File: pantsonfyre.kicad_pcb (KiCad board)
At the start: 2 copper layers, 27 parts, among them J1 3.5mm TRRS, J2 USB_C_Receptacle, SW1 SW_Push, SW2 SW_Push, SW3 SW_Push, U1 CAP1206-x-SL, U2 STM32C011J4Mx, U3 MCP4725xxx-xCH, U4 CAP1206-x-SL, U5 CAP1206-x-SL, U7 AMS1117-3.3, U8 PAM8302AAD

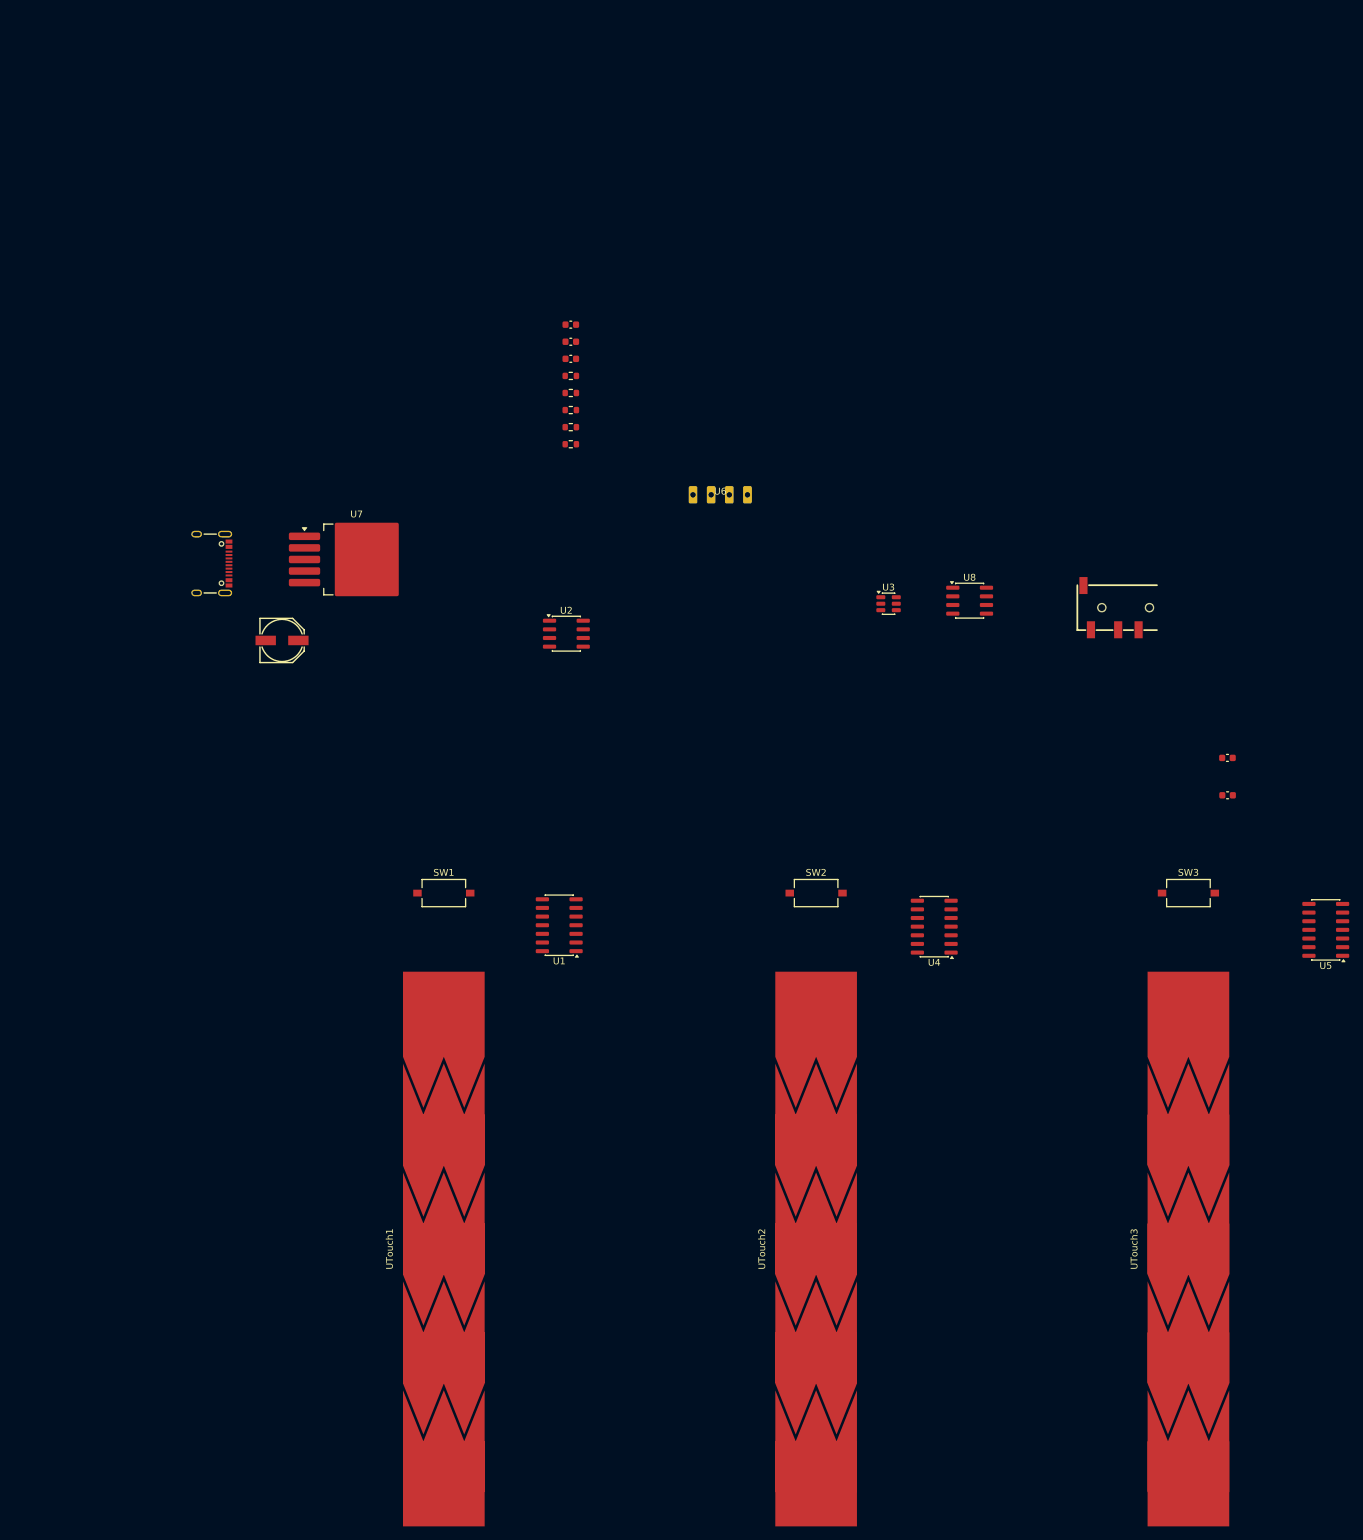
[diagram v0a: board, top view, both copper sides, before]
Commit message: Did lots of stuff + removed the custom footprint for header
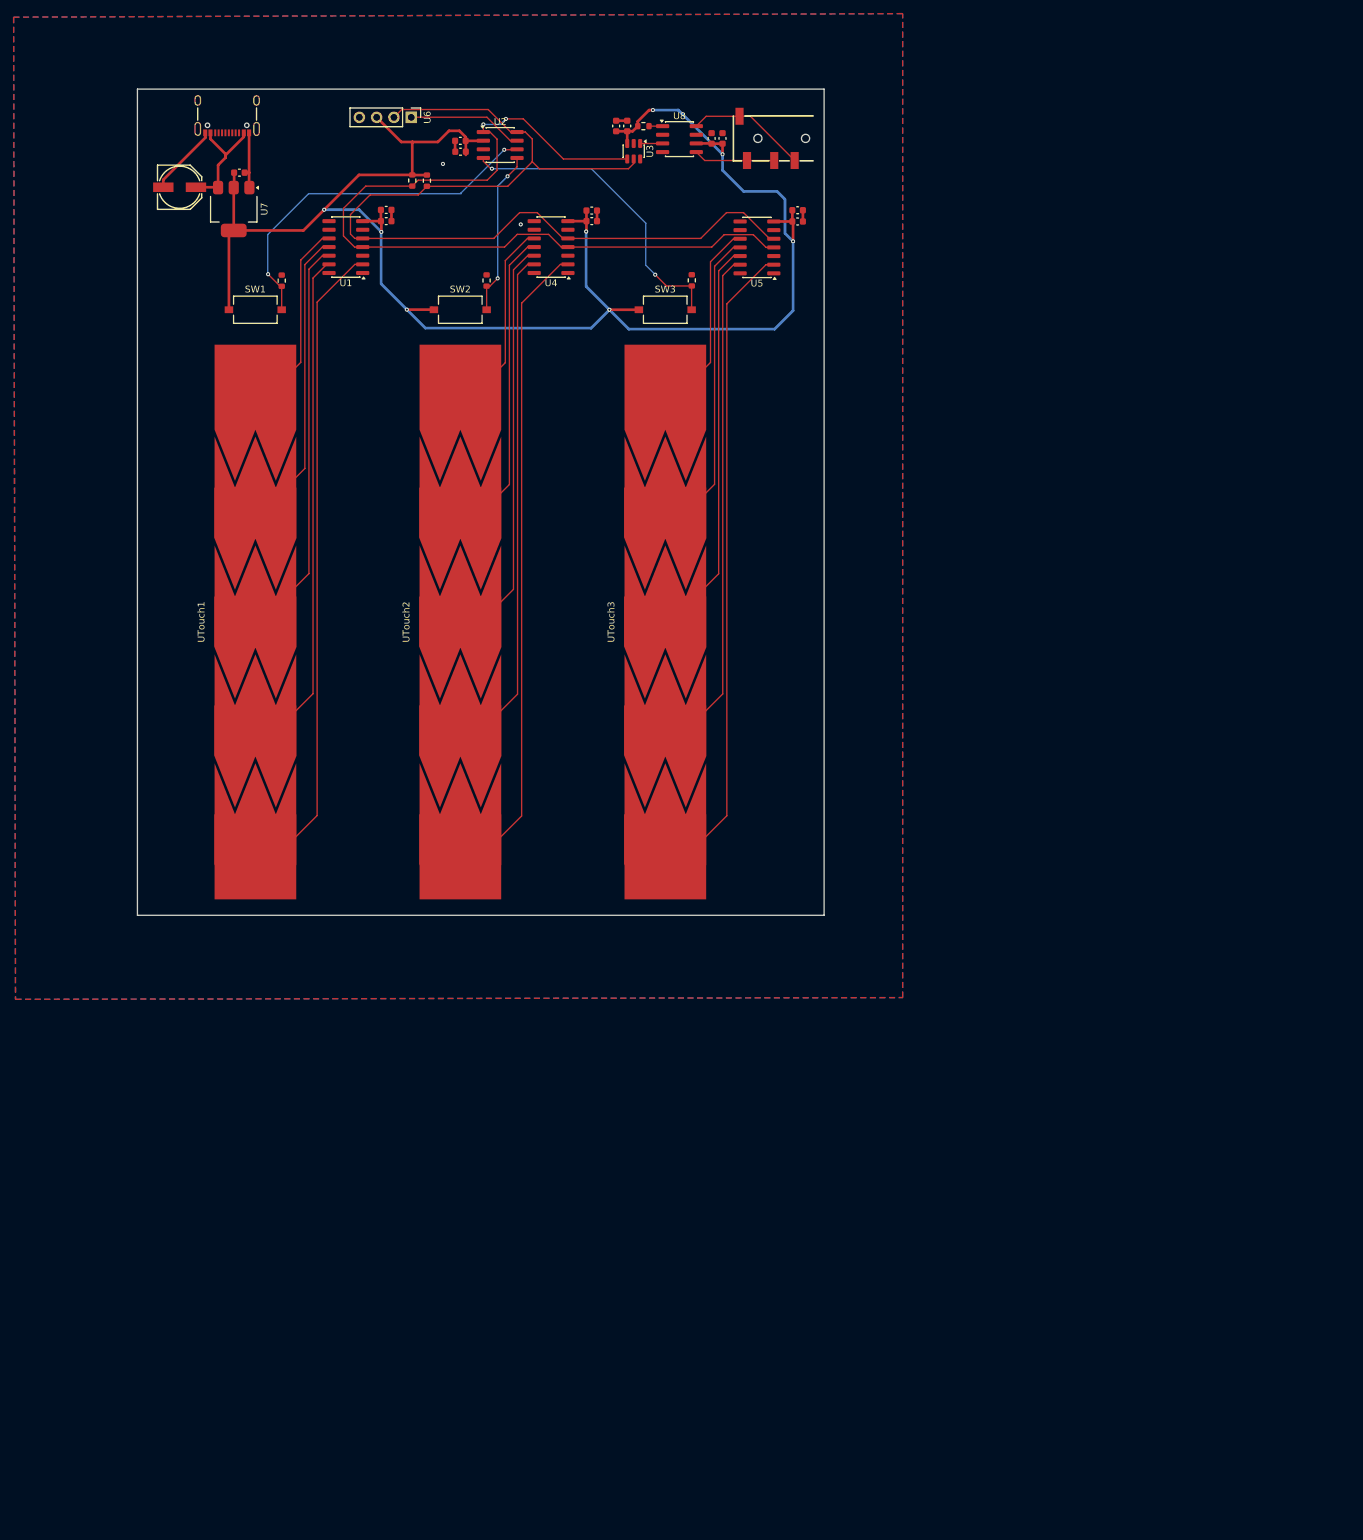
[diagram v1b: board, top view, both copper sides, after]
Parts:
- added C10: 0.1uF, PCM_SparkFun-Capacitor:C_0603_1608Metric, F.Cu at (136.7, 51.0)
- added C11: 0.1uF, PCM_SparkFun-Capacitor:C_0603_1608Metric, F.Cu at (166.9, 49.4)
- added C12: 1.0uF, PCM_SparkFun-Capacitor:C_0603_1608Metric, F.Cu at (166.9, 51.0)
- added C13: 0.1uF, PCM_SparkFun-Capacitor:C_0603_1608Metric, F.Cu at (197.1, 51.0)
- added C14: 1.0uF, PCM_SparkFun-Capacitor:C_0603_1608Metric, F.Cu at (197.1, 49.4)
- added C7: 10uF, PCM_SparkFun-Capacitor:C_0603_1608Metric, F.Cu at (170.4, 37.0)
- added C8: 1.0uF, PCM_SparkFun-Capacitor:C_0603_1608Metric, F.Cu at (172.1, 37.0)
- added C9: 1.0uF, PCM_SparkFun-Capacitor:C_0603_1608Metric, F.Cu at (136.7, 49.3)
- added R6: 10k, PCM_SparkFun-Resistor:R_0603_1608Metric, F.Cu at (174.4, 37.0)
- C6: value 0.1uF -> 1.0uF
- U6: footprint Slider:STLink-Headers -> Connector_PinHeader_2.54mm:PinHeader_1x04_P2.54mm_Vertical
- U7: footprint Package_TO_SOT_SMD:TO-263-5_TabPin3 -> Package_TO_SOT_SMD:SOT-223-3_TabPin2
- moved U5 130.5 mm to (191.1, 54.9)
- moved C6 121.7 mm to (186.1, 38.8), turned to 90 degrees
- moved UTouch3 120.0 mm to (177.7, 109.9)
- moved C5 118.4 mm to (184.5, 38.8), turned to 90 degrees
- moved SW3 115.1 mm to (177.7, 64.0)
- moved U4 114.6 mm to (160.9, 54.8)
- moved UTouch2 105.9 mm to (147.6, 109.9)
- moved U1 104.5 mm to (130.7, 54.8)
- moved SW2 100.4 mm to (147.5, 64.0)
- moved UTouch1 96.2 mm to (117.4, 109.9)
- moved SW1 90.1 mm to (117.4, 64.0)
- moved J1 85.5 mm to (194.8, 38.8)
- moved U8 80.1 mm to (179.7, 38.9)
- moved U3 76.3 mm to (173.0, 40.7), turned to -90 degrees
- moved U2 72.5 mm to (153.4, 39.8)
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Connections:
- net 5V renamed /+5V
- U8 pad 1: unconnected-(U8-~{SD}-Pad1) -> Net-(U8-~{SD})
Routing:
- net 3.3V: track 0.00 -> 260.7 mm, vias 0 -> 8
- net Net-(U1-SMCLK): track 0.00 -> 143.8 mm
- net Net-(U1-SMDATA): track 0.00 -> 128.2 mm, vias 0 -> 2
- net Net-(U5-CS1): track 0.00 -> 93.0 mm
- net Net-(U1-CS1): track 0.00 -> 93.0 mm
- net Net-(U4-CS1): track 0.00 -> 93.0 mm
- net Net-(U5-CS2): track 0.00 -> 72.4 mm
- net Net-(U4-CS2): track 0.00 -> 72.4 mm
- net Net-(U1-CS2): track 0.00 -> 72.0 mm
- net Net-(U4-CS3): track 0.00 -> 57.6 mm
- net Net-(U2-PA10/PA12): track 0.00 -> 53.9 mm, vias 0 -> 2
- net Net-(U5-CS3): track 0.00 -> 53.3 mm
- net Net-(U1-CS3): track 0.00 -> 53.3 mm
- net Net-(U2-PA0/PA1/PA2/PF2): track 0.00 -> 45.8 mm, vias 0 -> 2
- net Net-(U5-CS4): track 0.00 -> 42.9 mm
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- added copper zone on B.Cu, net GND
- added copper zone on F.Cu, net GND
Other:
- board outline added: 100.9 x 121.4 mm
